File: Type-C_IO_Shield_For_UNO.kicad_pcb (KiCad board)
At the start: 2 copper layers, 68.6 x 53.3 mm, 44 parts, among them J1 Conn_01x04, J10 Conn_01x04, J11 Conn_01x04, J12 Conn_01x04, J13 Conn_01x04, J14 Conn_01x04, J15 Conn_01x04, J17 Conn_01x06, J18 Conn_01x06, J19 Conn_01x06, J2 Conn_01x04, J21 Conn_01x04, J22 Conn_01x04, J23 Conn_01x04, J24 Conn_01x04, J25 Conn_01x04, J26 Conn_01x06, J27 Conn_01x06, J28 Screw_Terminal_01x02, J3 Conn_01x04, J4 USB_C_Receptacle_USB2.0, J5 Conn_01x04, J6 Conn_01x04, J7 Conn_01x04, P1 Power, P2 Analog, P3 Digital, P4 Digital, P5 CONN_01X01, P6 CONN_01X01, P7 CONN_01X01, P8 CONN_01X01, SW1 SW_SPST, U1 CH340C

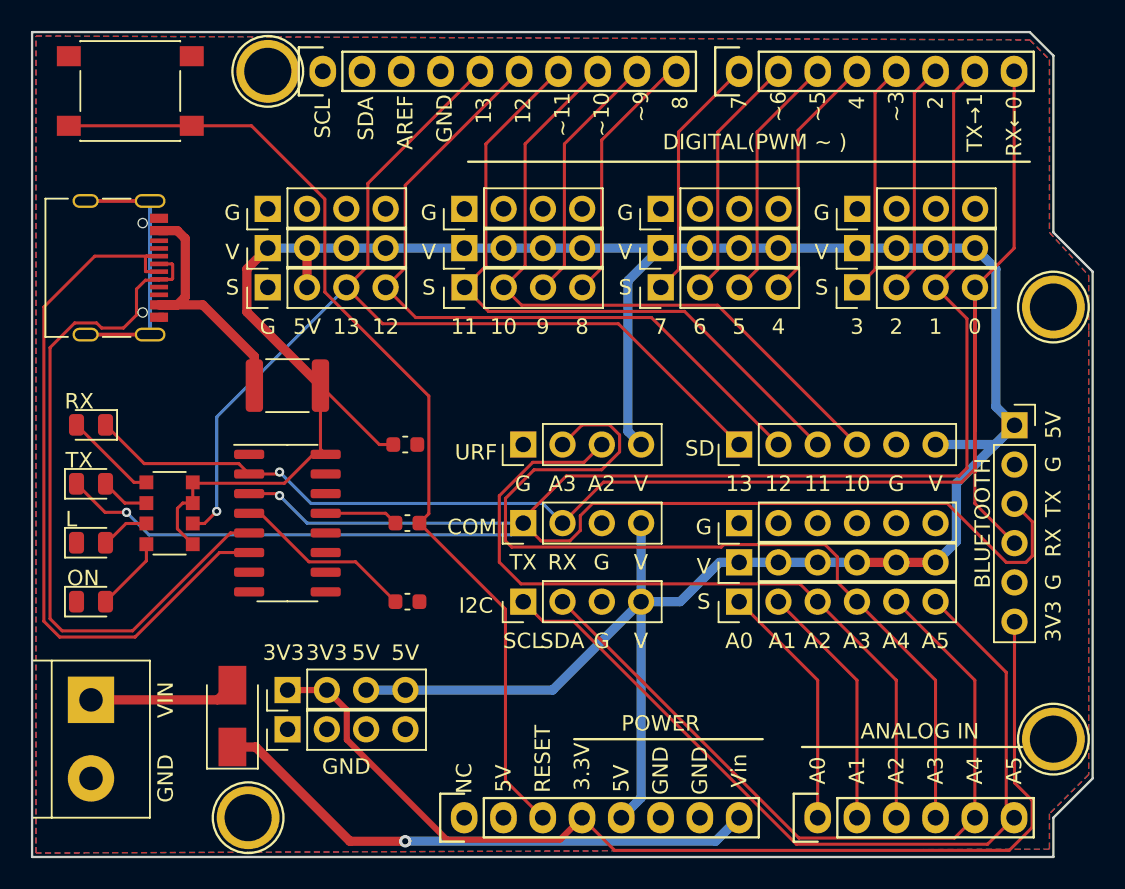
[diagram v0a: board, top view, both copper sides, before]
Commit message: V1.2
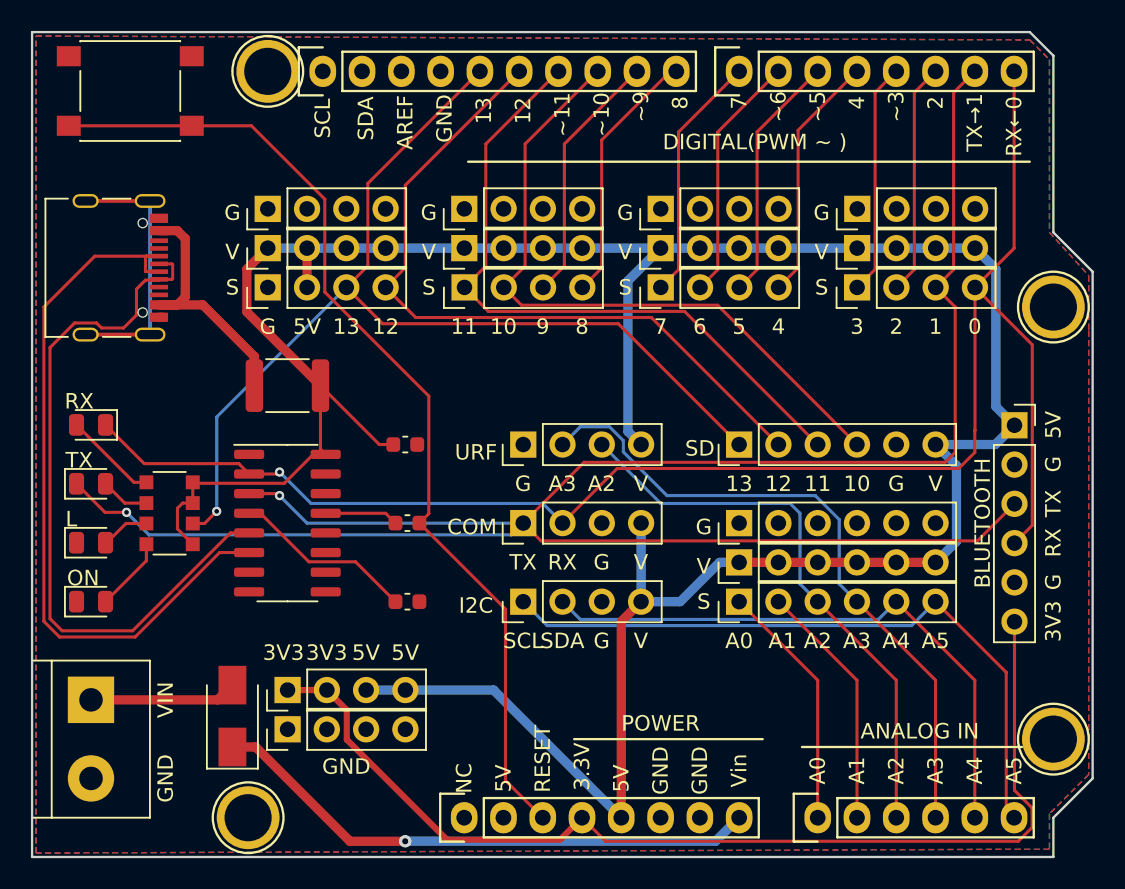
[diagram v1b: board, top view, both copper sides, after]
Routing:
- net /A3: track 58.5 -> 43.1 mm
- net /A2: track 50.0 -> 36.9 mm
- net /A4(SDA): track 49.6 -> 38.6 mm
- net /A5(SCL): track 55.0 -> 44.0 mm
- net /1(Tx): track 147.5 -> 138.3 mm
- net +5V: track 187.9 -> 185.4 mm
